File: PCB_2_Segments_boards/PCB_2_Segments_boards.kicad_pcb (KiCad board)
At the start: 2 copper layers, 4 parts

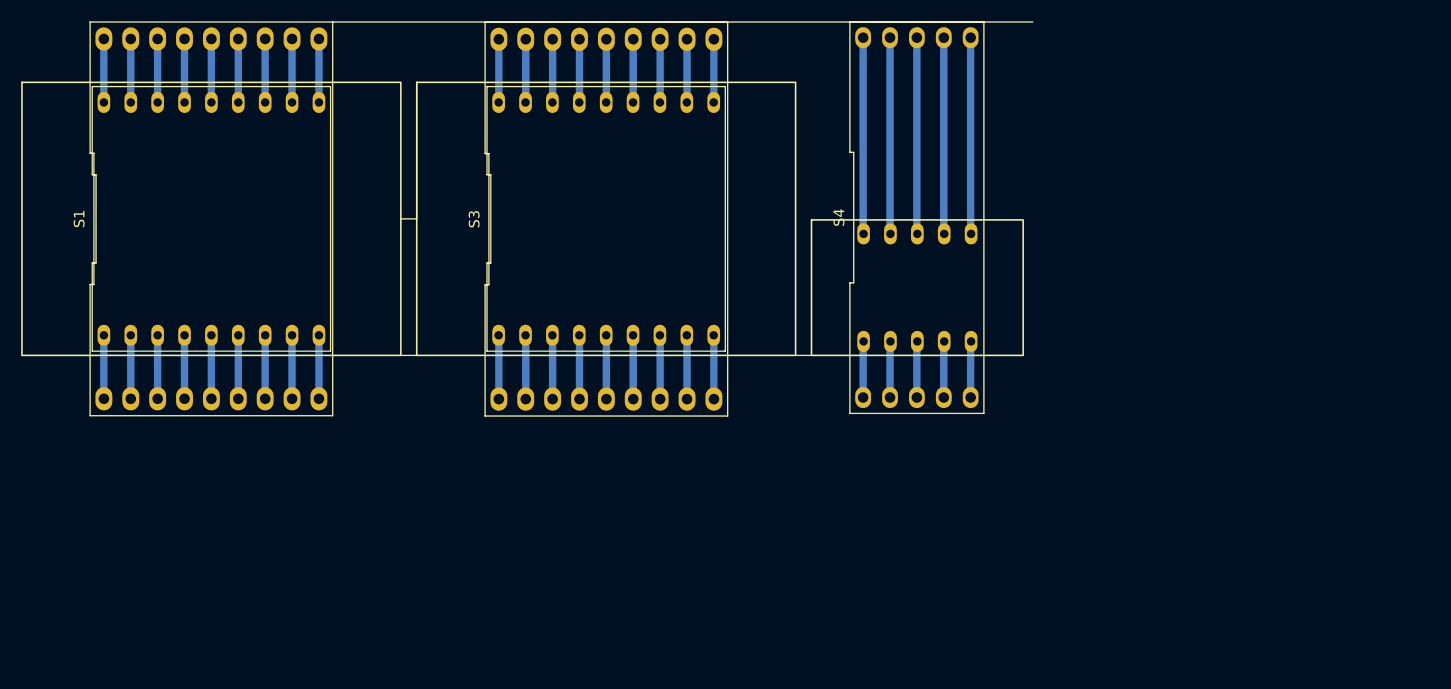
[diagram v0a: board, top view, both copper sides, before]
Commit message: backup update
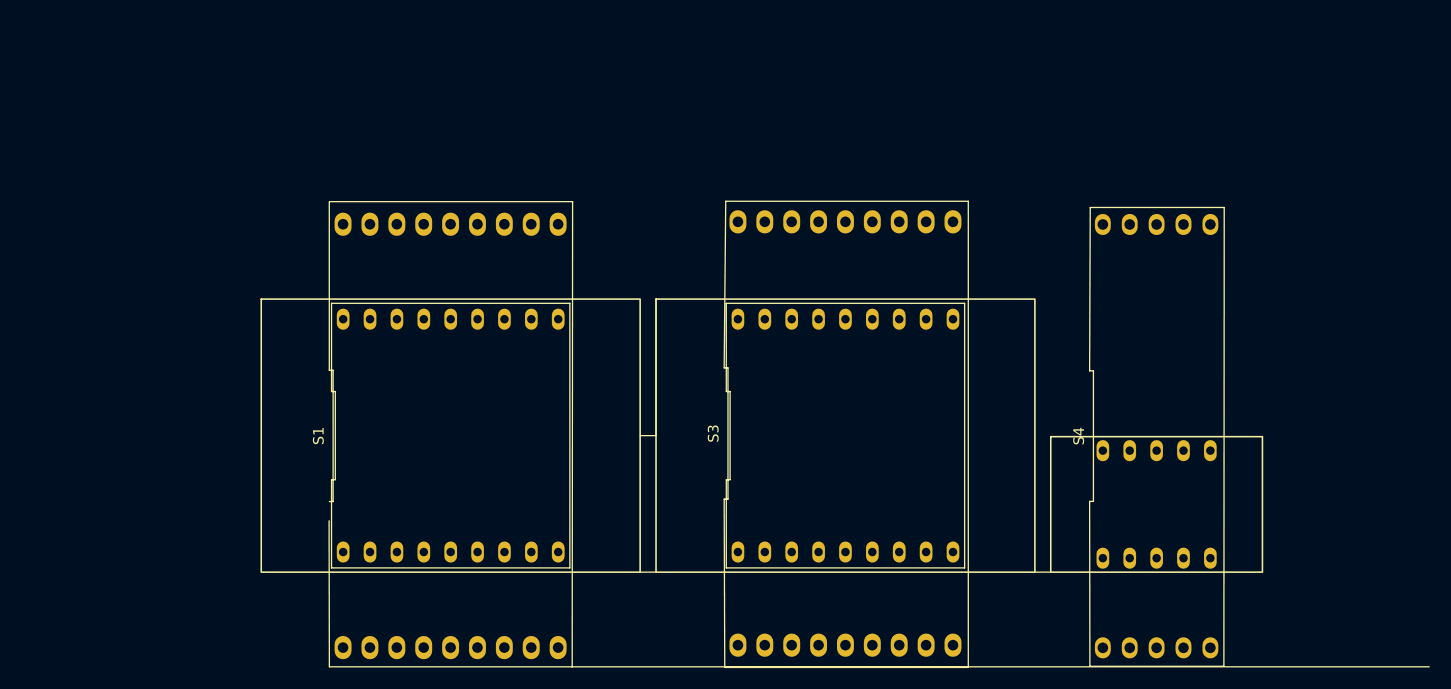
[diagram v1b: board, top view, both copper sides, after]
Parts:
- moved S4 30.7 mm to (189.5, 102.0)
- moved S1 30.5 mm to (122.8, 102.0)
- moved S2 30.5 mm to (122.8, 102.0)
- moved S3 30.3 mm to (160.1, 101.8)
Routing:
- net Net-(S2-Pad25): track 18.6 -> 0.00 mm
- net Net-(S2-Pad24): track 18.6 -> 0.00 mm
- net Net-(S2-Pad23): track 18.6 -> 0.00 mm
- net Net-(S2-Pad22): track 18.6 -> 0.00 mm
- net Net-(S2-Pad19): track 18.6 -> 0.00 mm
- net Net-(S1-Pad40): track 6.38 -> 0.00 mm
- net Net-(S2-Pad33): track 6.04 -> 0.00 mm
- net Net-(S2-Pad30): track 6.04 -> 0.00 mm
- net Net-(S2-Pad18): track 6.04 -> 0.00 mm
- net Net-(S2-Pad13): track 6.04 -> 0.00 mm
- net Net-(S2-Pad15): track 6.04 -> 0.00 mm
- net Net-(S2-Pad34): track 6.04 -> 0.00 mm
- net Net-(S2-Pad32): track 6.04 -> 0.00 mm
- net Net-(S2-Pad29): track 6.04 -> 0.00 mm
- net Net-(S2-Pad14): track 6.04 -> 0.00 mm
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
